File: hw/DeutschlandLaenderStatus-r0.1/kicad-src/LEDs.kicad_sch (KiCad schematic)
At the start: 16 parts

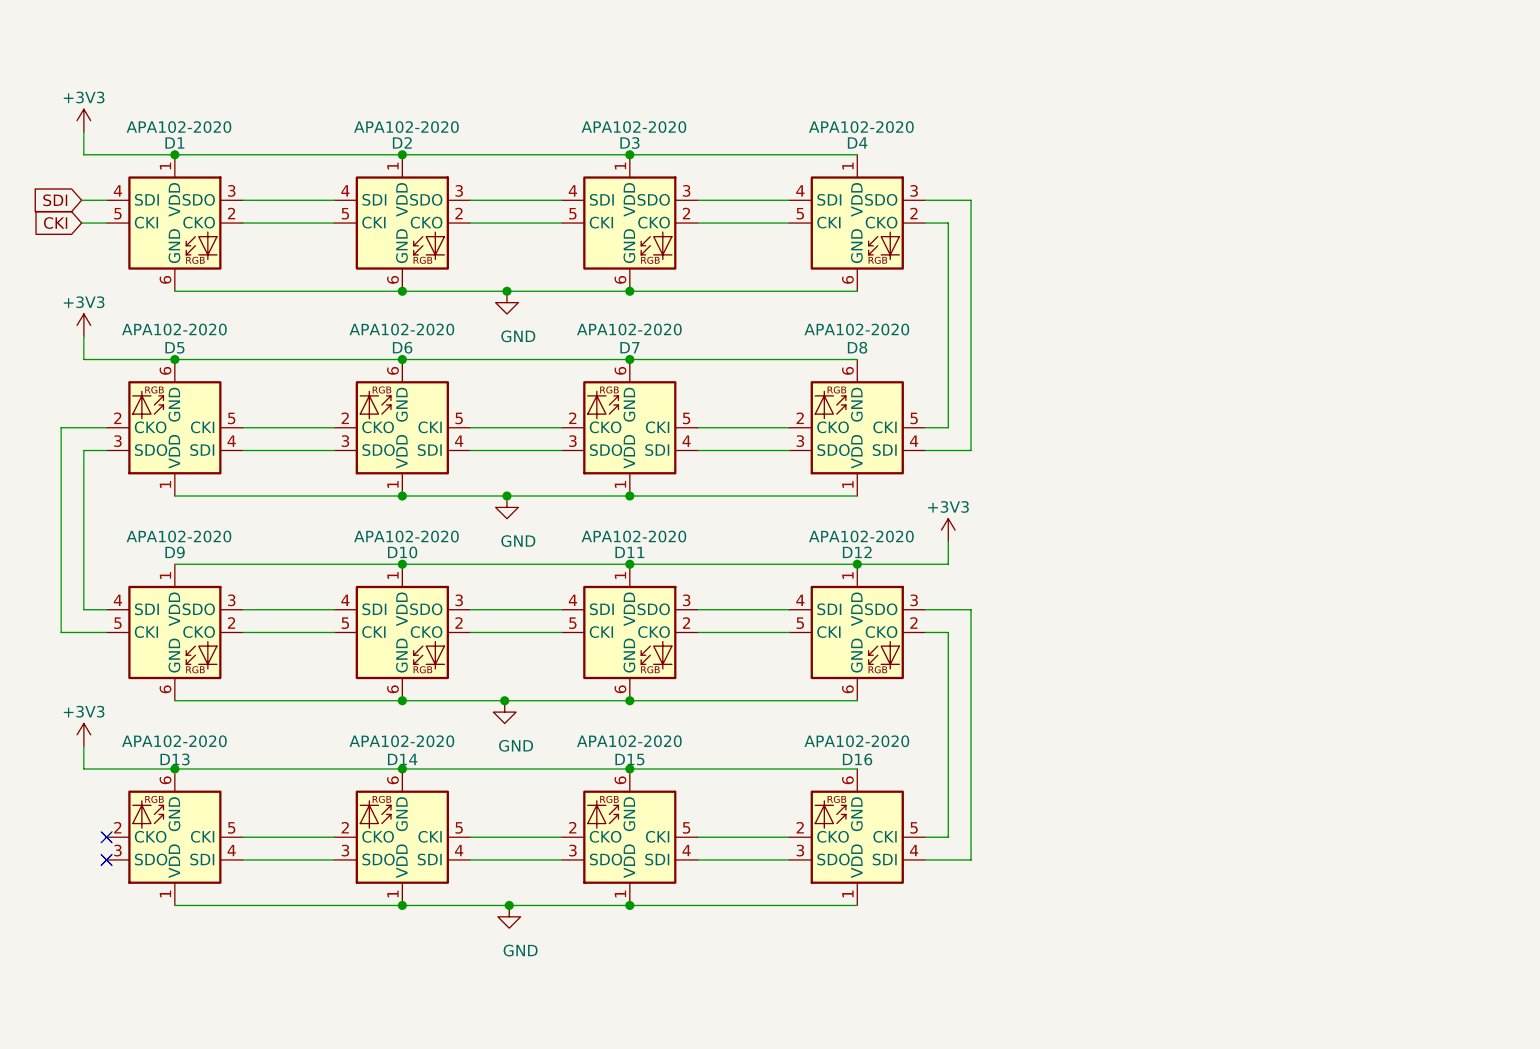
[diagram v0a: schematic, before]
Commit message: Layout complete
Need to added Map Outline still
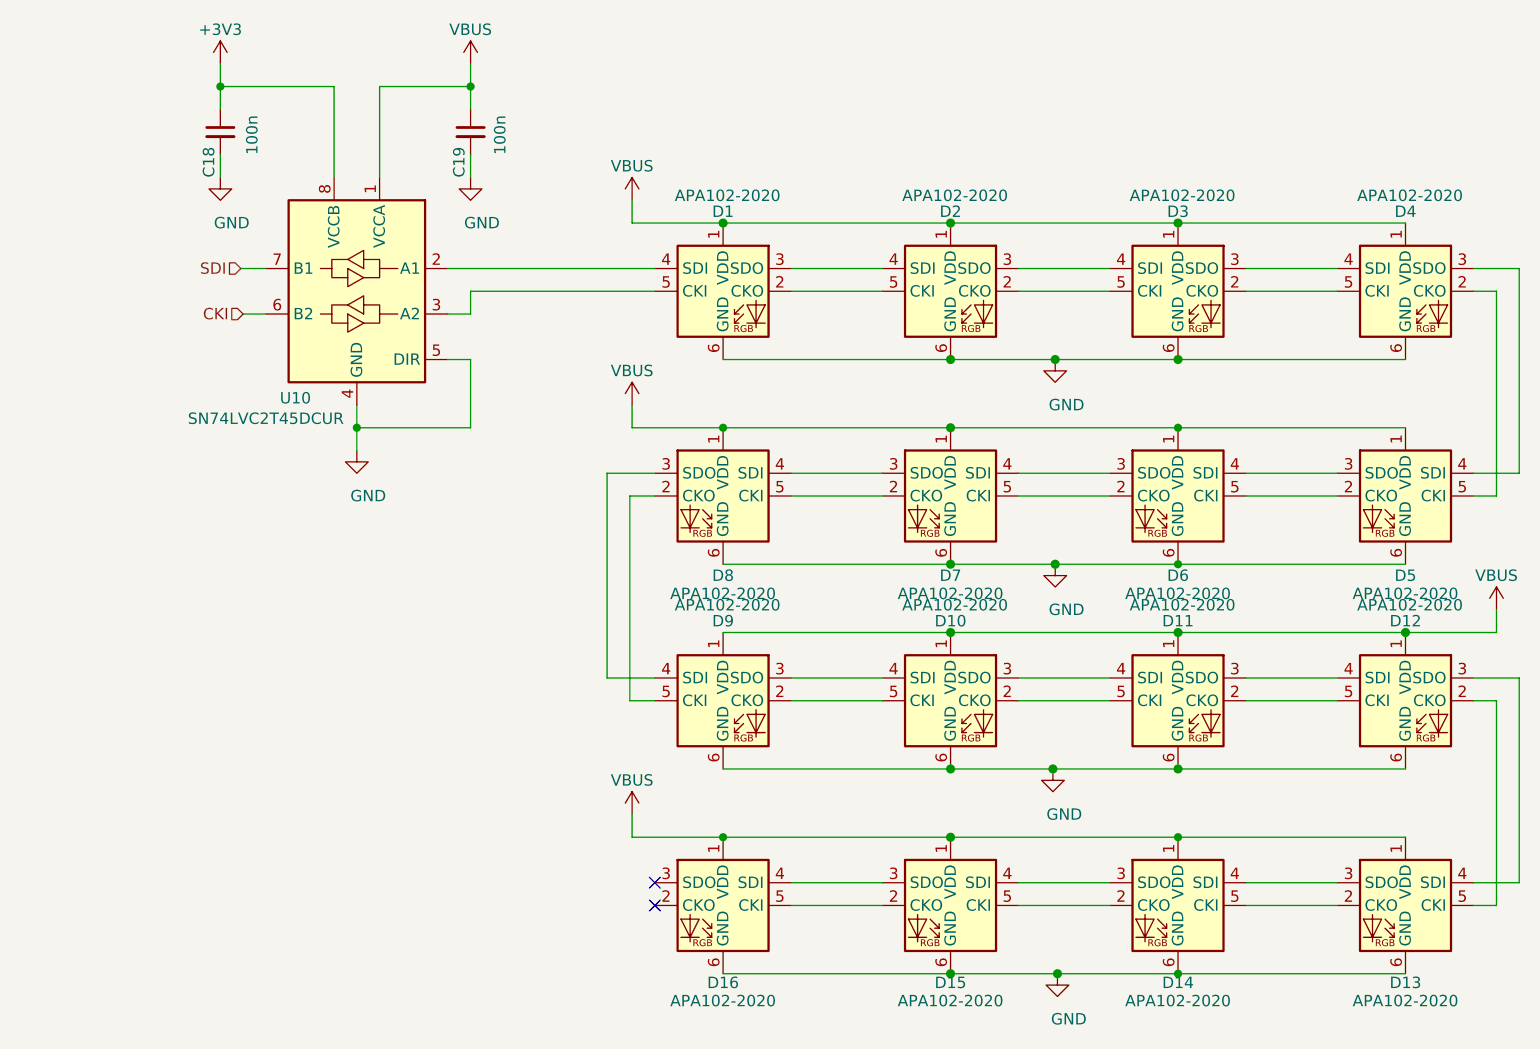
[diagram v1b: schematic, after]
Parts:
- added C18, C19: 100n, Capacitor_SMD:C_0402_1005Metric, symbol icebreaker-bitsy-rescue:pkl_C_Small-pkl_device
- added U10: SN74LVC2T45DCUR, Package_SO:VSSOP-8_2.4x2.1mm_P0.5mm, symbol Logic_LevelTranslator:SN74LVC2T45DCUR
- D1, D10, D11, D12, D13, D14, D15, D16, D2, D3, D4, D5, D6, D7, D8, D9: footprint LED_SMD:LED-APA102-2020 -> kt-footprints:LED-APA102-2020
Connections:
- net +3V3: now also C18.1, U10.8 (VCCB); no longer D1.1 (VDD), D10.1 (VDD), D11.1 (VDD), D12.1 (VDD), D13.6 (GND), D14.6 (GND), D15.6 (GND), D16.6 (GND), D2.1 (VDD), D3.1 (VDD), D4.1 (VDD), D5.6 (GND), D6.6 (GND), D7.6 (GND), D8.6 (GND), D9.1 (VDD)
- net CKI: now also U10.6 (B2); no longer D1.5 (CKI)
- net GND: now also D13.6 (GND), D14.6 (GND), D15.6 (GND), D16.6 (GND), D5.6 (GND), D6.6 (GND), D7.6 (GND), D8.6 (GND), C18.2, C19.2, U10.4 (GND), U10.5 (DIR); no longer D13.1 (VDD), D14.1 (VDD), D15.1 (VDD), D16.1 (VDD), D5.1 (VDD), D6.1 (VDD), D7.1 (VDD), D8.1 (VDD)
- net SDI: now also U10.7 (B1); no longer D1.4 (SDI)
- net at D14.2 (CKO): now also D15.5 (CKI); no longer D13.5 (CKI)
- net at D14.3 (SDO): now also D15.4 (SDI); no longer D13.4 (SDI)
- net at D14.4 (SDI): now also D13.3 (SDO); no longer D15.3 (SDO)
- net at D14.5 (CKI): now also D13.2 (CKO); no longer D15.2 (CKO)
- net at D4.2 (CKO): now also D5.5 (CKI); no longer D8.5 (CKI)
- net at D4.3 (SDO): now also D5.4 (SDI); no longer D8.4 (SDI)
- net at D7.2 (CKO): now also D8.5 (CKI); no longer D6.5 (CKI)
- net at D7.3 (SDO): now also D8.4 (SDI); no longer D6.4 (SDI)
- net at D7.4 (SDI): now also D6.3 (SDO); no longer D8.3 (SDO)
- net at D7.5 (CKI): now also D6.2 (CKO); no longer D8.2 (CKO)
- net at D12.2 (CKO): now also D13.5 (CKI); no longer D16.5 (CKI)
- net at D12.3 (SDO): now also D13.4 (SDI); no longer D16.4 (SDI)
- net at D9.4 (SDI): now also D8.3 (SDO); no longer D5.3 (SDO)
- net at D9.5 (CKI): now also D8.2 (CKO); no longer D5.2 (CKO)
- net at D16.2 (CKO): no longer D15.5 (CKI)
- net at D16.3 (SDO): no longer D15.4 (SDI)
- new net: D1.4 (SDI), U10.2 (A1)
- new net: D1.5 (CKI), U10.3 (A2)
- new net: D15.3 (SDO), D16.4 (SDI)
- new net: D15.2 (CKO), D16.5 (CKI)
- new net: D5.2 (CKO), D6.5 (CKI)
- new net: D5.3 (SDO), D6.4 (SDI)
- new net VBUS: C19.1, D1.1 (VDD), D10.1 (VDD), D11.1 (VDD), D12.1 (VDD), D13.1 (VDD), D14.1 (VDD), D15.1 (VDD), D16.1 (VDD), D2.1 (VDD), D3.1 (VDD), D4.1 (VDD), D5.1 (VDD), D6.1 (VDD), D7.1 (VDD), D8.1 (VDD), D9.1 (VDD), U10.1 (VCCA)
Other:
- moved on the sheet: D1, D10, D11, D12, D13, D14, D15, D16, D2, D3, D4, D5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
